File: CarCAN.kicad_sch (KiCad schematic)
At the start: 10 parts, among them IC1 TCAN337DCNR, U3 CDSOT23-T24CAN

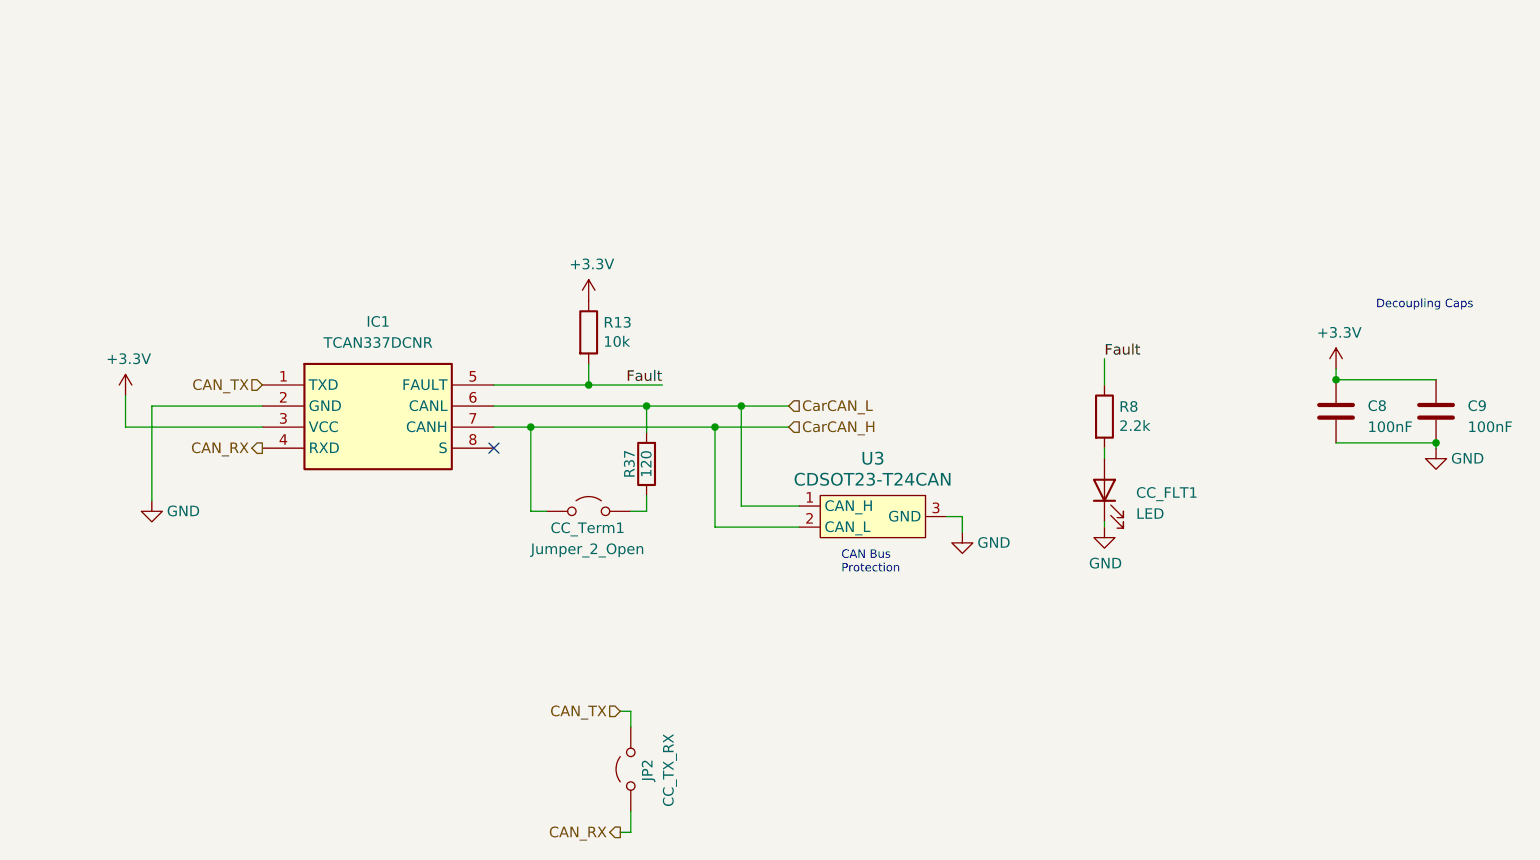
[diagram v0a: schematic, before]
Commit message: MCU pins, PSON power distribution, KiCad-Sharepoint, and 7 seg
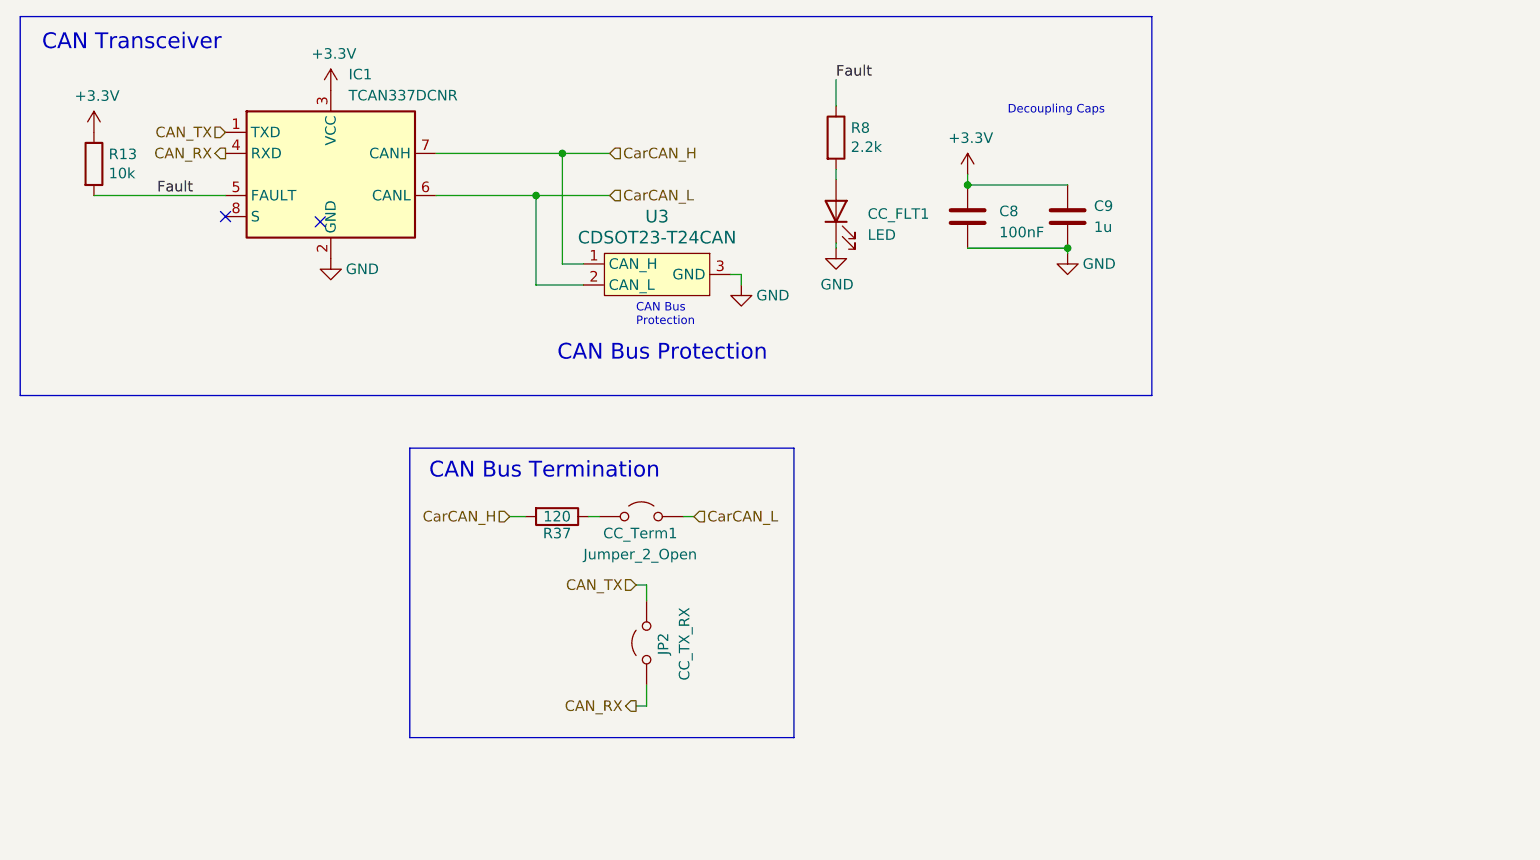
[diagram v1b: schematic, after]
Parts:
- C9: value 100nF -> 1u
- IC1: footprint UTSVT_ICs:SOT65P280X145-8N -> UTSVT_ICs:TCAN337DCNR; symbol utsvt-chips:TCAN337DCNR -> UTSVT-ICs:TCAN337; P/N (none) -> TCAN337DCNR
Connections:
- net CarCAN_H: now also R37.2, U3.1 (CAN_H); no longer CC_Term1.1 (A), U3.2 (CAN_L)
- net CarCAN_L: now also CC_Term1.2 (B), U3.2 (CAN_L); no longer R37.2, U3.1 (CAN_H)
- net at R37.1: now also CC_Term1.1 (A); no longer CC_Term1.2 (B)
- no-connect marks 1 -> 2
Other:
- note added: "CAN Bus Termination"
- note added: "CAN Transceiver"
- moved on the sheet: C8, C9, CC_FLT1, CC_Term1, IC1, JP2, R13, R37, R8, U3
